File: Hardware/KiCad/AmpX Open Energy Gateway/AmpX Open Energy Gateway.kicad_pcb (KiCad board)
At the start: 2 copper layers, 33 x 85 mm, 4 parts, among them U1 ESP32-DevKitC

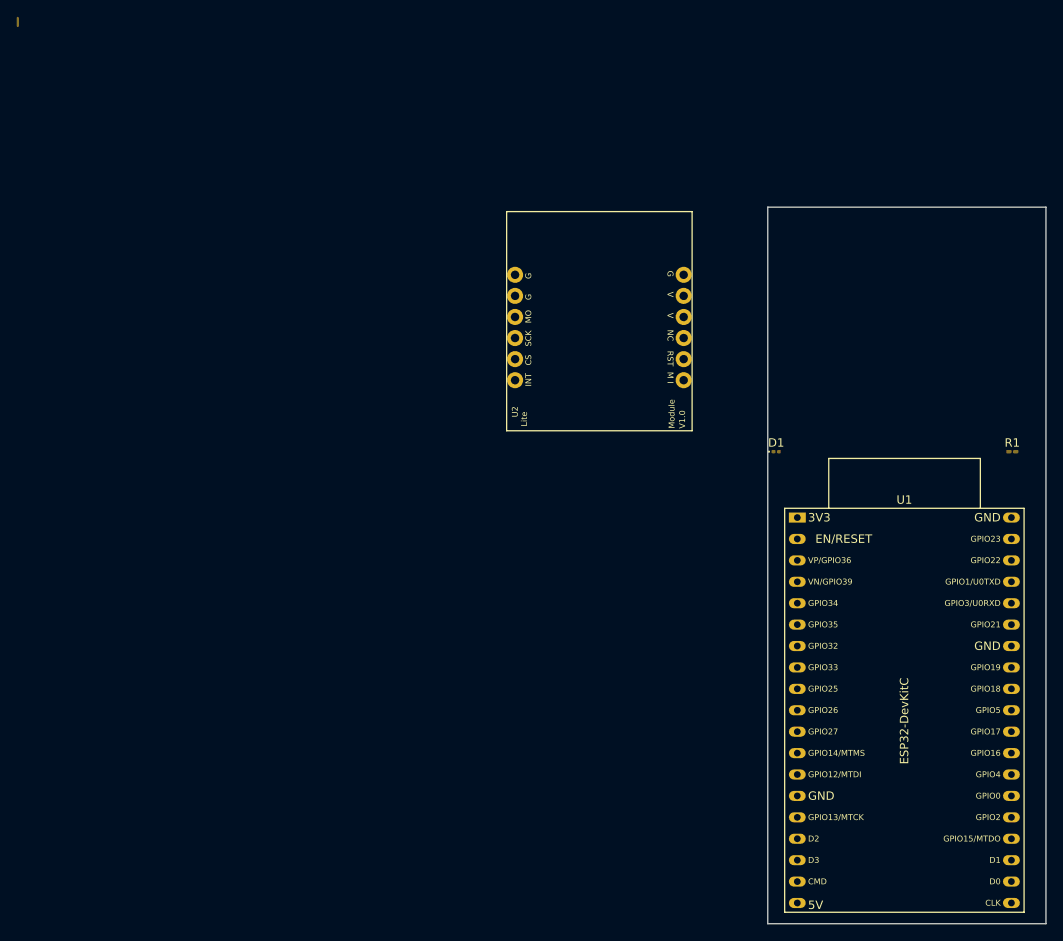
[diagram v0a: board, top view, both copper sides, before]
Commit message: updated schmatic, and pcb
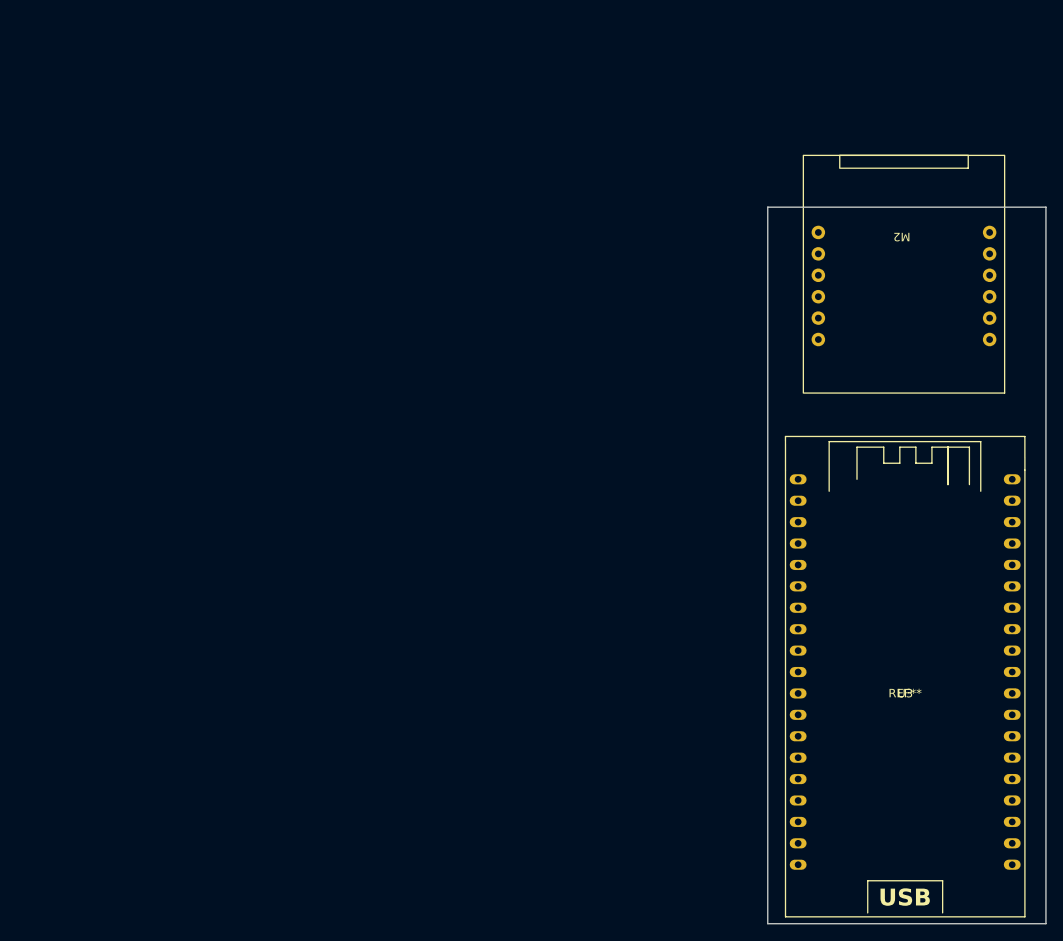
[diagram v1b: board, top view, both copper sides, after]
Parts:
- removed D1: LED, LED_SMD:LED_0201_0603Metric
- removed R1: R, Resistor_SMD:R_0201_0603Metric_Pad0.64x0.40mm_HandSolder
- removed U1: ESP32-DevKitC, PCM_Espressif:ESP32-DevKitC
- removed U2: ~, AmpX-Footprint-Library.pretty:W5500-Lite-Module
- added M2: ~, Module_Ethernet_LAN_W5500_Lite.3dshapes:Module_Ethernet_LAN_W5500_Lite, F.Cu at (105.3, 31.0)
- added U3: Module_MCU_ESP32_WROOM32_38PINS, Module_MCU_ESP32_WROOM32_38PINS:Module_MCU_ESP32_WROOM32_38PINS_HEADERPINS, F.Cu at (82.6, 60.3)
